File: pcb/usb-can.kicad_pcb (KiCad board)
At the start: 4 copper layers, 48.8 x 33 mm, 54 parts, among them J1 Micro_SD_Card_Det1, J2 Conn_ARM_SWD_TagConnect_TC203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, J3 USB_C_Receptacle_USB2.0_16P, J4 Conn_01x04_MountingPin, J5 Conn_01x04_MountingPin, U1 STM32G473CBTx, U2 TJA1042T-3, U3 SRV05-4, U4 AMS1117-3.3, U5 TPS5430DDA, Y1 16MHz

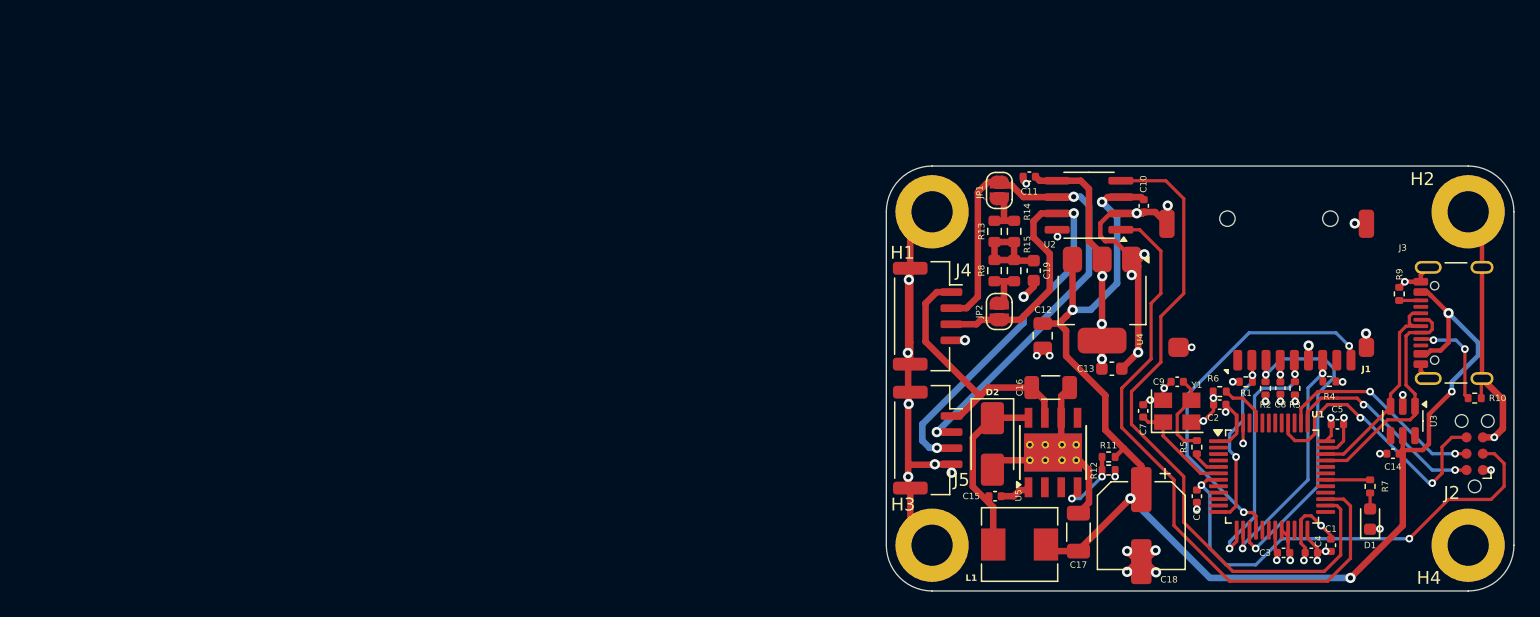
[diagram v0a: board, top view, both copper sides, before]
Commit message: Finish rev2
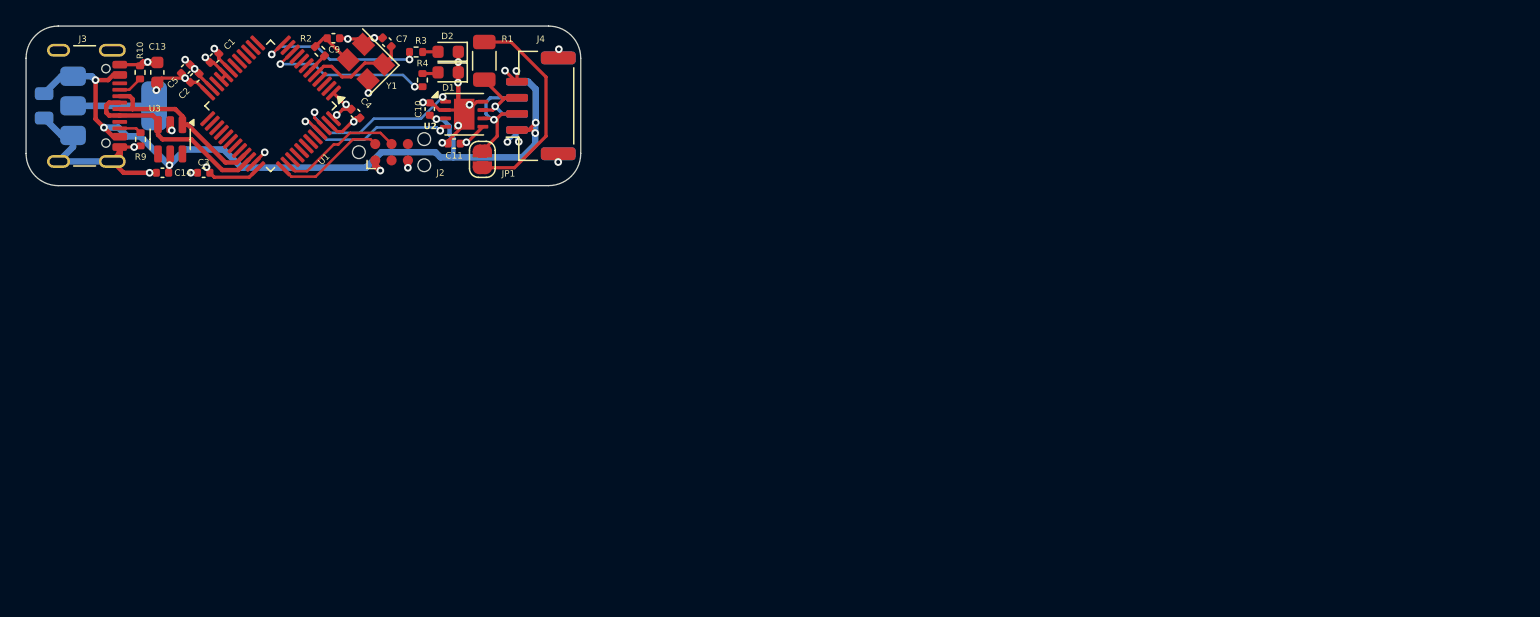
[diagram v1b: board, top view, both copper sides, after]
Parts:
- removed C15: 10n, Capacitor_SMD:C_0402_1005Metric
- removed C16, C17: 22u, Capacitor_SMD:C_1206_3216Metric
- removed C18: 220u, Capacitor_SMD:CP_Elec_6.3x5.4
- removed C19: 1n, Capacitor_SMD:C_0603_1608Metric
- removed C6, C8: 100n, Capacitor_SMD:C_0402_1005Metric
- removed H1, H2, H3, H4: MountingHole_Pad, MountingHole:MountingHole_3.2mm_M3_ISO7380_Pad
- removed J1: Micro_SD_Card_Det1, User_Footprints:SD-CARD
- removed JP2: SolderJumper_2_Open, Jumper:SolderJumper-2_P1.3mm_Open_RoundedPad1.0x1.5mm
- removed L1: 15u, Inductor_SMD:L_Sunlord_MWSA0503S
- removed R11, R6: 10k, Resistor_SMD:R_0402_1005Metric
- removed R12: 3k3, Resistor_SMD:R_0402_1005Metric
- removed R13, R14, R15, R8: 120, Resistor_SMD:R_0603_1608Metric
- removed R5, R7: 510, Resistor_SMD:R_0402_1005Metric
- removed U5: TPS5430DDA, Package_SO:TI_SO-PowerPAD-8_ThermalVias
- C12, J5, U4: moved to B.Cu
- C7, C9: value 10p -> 12p
- D1: value LEDB -> LEDR
- D2: value SS34 -> GLED; footprint Diode_SMD:D_SMA -> LED_SMD:LED_0603_1608Metric
- R1: value 10k -> 120; footprint Resistor_SMD:R_0402_1005Metric -> Resistor_SMD:R_1206_3216Metric
- R2, R3, R4: value 10k -> 1k
- U2: value TJA1042T-3 -> TJA1044GTK/3; footprint Package_SO:SOIC-8_3.9x4.9mm_P1.27mm -> Package_SON:HVSON-8-1EP_3x3mm_P0.65mm_EP1.6x2.4mm
- moved J3 109.8 mm to (85.6, 70.0), turned to -90 degrees
- moved R10 106.8 mm to (90.9, 67.4), turned to 90 degrees
- moved R9 98.5 mm to (90.9, 72.6), turned to -90 degrees
- moved U3 98.2 mm to (93.2, 72.6)
- moved C14 98.1 mm to (92.6, 75.2)
- moved C1 94.6 mm to (96.6, 66.3), turned to 45 degrees
- moved C5 93.6 mm to (94.4, 67.1), turned to 45 degrees
- moved C3 89.0 mm to (95.8, 75.2)
- moved J2 87.4 mm to (110.4, 73.6), turned to 0 degrees
- moved C2 83.6 mm to (95.1, 67.8), turned to 45 degrees
- moved U1 83.0 mm to (101.0, 70.0), turned to -135 degrees
- moved C4 81.7 mm to (107.6, 70.6), turned to -45 degrees
- moved C12 79.6 mm to (83.4, 70.0)
- moved D1 79.6 mm to (114.8, 67.4), turned to 180 degrees
- moved U4 78.3 mm to (88.8, 70.0), turned to 0 degrees
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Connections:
- C7 pad 2: /XTALO -> /XTALI
- D2 pad 1: Net-(D2-K) -> GND
- D2 pad 2: GND -> Net-(D2-A)
- J2 pad 3: /RST -> unconnected-(J2-~{RESET}-Pad3)
- J2 pad 6: /SWO -> unconnected-(J2-SWO-Pad6)
- J4 pad 1: +12V -> +5V
- J5 pad 1: +12V -> +5V
- R1 pad 1: +3V3 -> /CANH
- R1 pad 2: /CS -> Net-(JP1-B)
- R2 pad 1: +3V3 -> /XTALR
- R2 pad 2: /MOSI -> /XTALO
- R3 pad 1: +3V3 -> /LEDG
- R3 pad 2: /SCK -> Net-(D2-A)
- R4 pad 1: +3V3 -> /LEDR
- R4 pad 2: /MISO -> Net-(D1-A)
- U1 pad 10: unconnected-(U1-PA2-Pad10) -> /LEDR
- U1 pad 12: /CS -> /LEDG
- U1 pad 13: /SCK -> unconnected-(U1-PA5-Pad13)
- U1 pad 14: /MISO -> unconnected-(U1-PA6-Pad14)
- U1 pad 15: /MOSI -> unconnected-(U1-PA7-Pad15)
- U1 pad 16: /DET -> unconnected-(U1-PB0-Pad16)
- U1 pad 26: /CNRX -> unconnected-(U1-PB12-Pad26)
- U1 pad 27: /CNTX -> unconnected-(U1-PB13-Pad27)
- U1 pad 30: /LEDB -> unconnected-(U1-PA8-Pad30)
- U1 pad 40: /SWO -> unconnected-(U1-PB3-Pad40)
- U1 pad 45: /BOOT0 -> /CNRX
- U1 pad 46: unconnected-(U1-PB9-Pad46) -> /CNTX
- U1 pad 7: /RST -> unconnected-(U1-PG10-Pad7)
- Y1 pad 1: /XTALO -> /XTALI
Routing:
- net GND: track 144.4 -> 56.2 mm, vias 42 -> 26
- net /CNRX: track 53.1 -> 13.6 mm, vias 0 -> 2
- net +5V: track 102.7 -> 64.9 mm
- net /RST: track 36.9 -> 0.00 mm, vias 2 -> 0
- net /CNTX: track 50.5 -> 14.0 mm, vias 0 -> 2
- net /CANH: track 43.1 -> 7.14 mm, vias 2 -> 1
- net /CANL: track 43.9 -> 10.1 mm, vias 2 -> 1
- net /DET: track 29.3 -> 0.00 mm, vias 2 -> 0
- net /MOSI: track 26.0 -> 0.00 mm, vias 2 -> 0
- net /SWO: track 22.0 -> 0.00 mm, vias 2 -> 0
- net +12V: track 21.3 -> 0.00 mm
- net /SCK: track 20.2 -> 0.00 mm, vias 2 -> 0
- net /MISO: track 19.3 -> 0.00 mm, vias 2 -> 0
- net /CS: track 14.9 -> 0.00 mm, vias 2 -> 0
- net Net-(D2-K): track 14.5 -> 0.00 mm
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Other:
- board size 48.8 x 33 mm -> 43.1 x 12.4 mm
